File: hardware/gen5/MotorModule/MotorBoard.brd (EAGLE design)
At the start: 61 x 50.1 mm, 42 parts, among them J1 M20X2SHROUDED

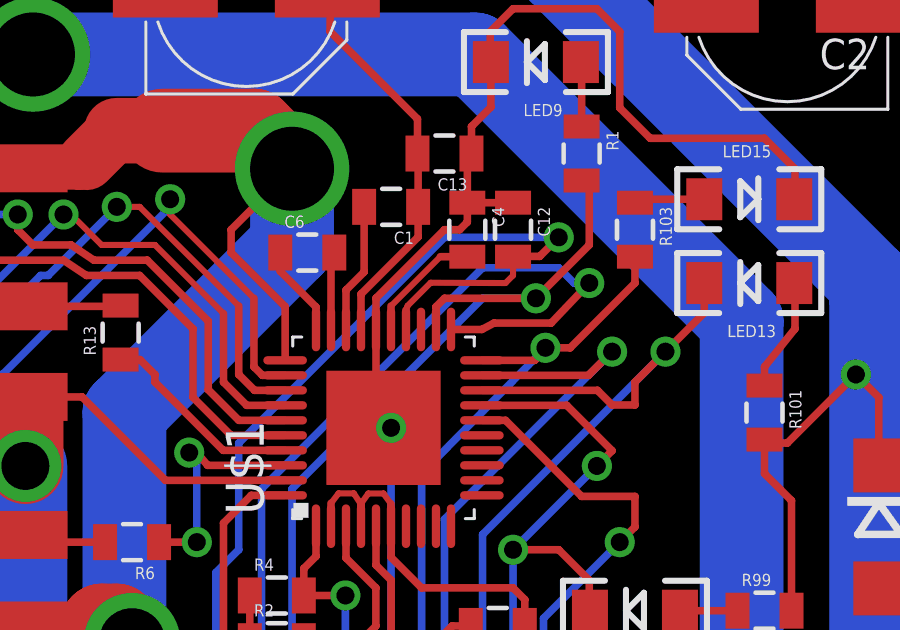
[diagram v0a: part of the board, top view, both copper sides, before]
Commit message: small tweak to motorboard
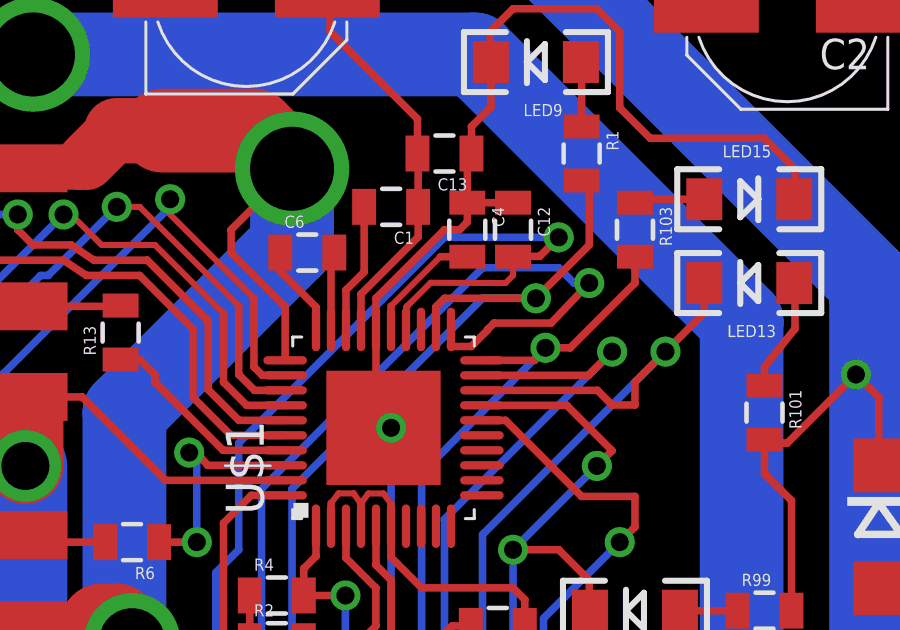
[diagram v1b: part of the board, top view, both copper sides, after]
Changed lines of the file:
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@@
 <wire x1="16.51" y1="36.83" x2="16.51" y2="42.672" width="3.81" layer="1"/>
 <via x="16.51" y="42.672" extent="1-16" drill="2.8"/>
-<wire x1="41.16" y1="33.759" x2="41.16" y2="34.937" width="0.254" layer="1"/>
 <wire x1="41.16" y1="34.937" x2="43.064" y2="36.841" width="0.254" layer="1"/>
 <wire x1="43.064" y1="36.841" x2="43.064" y2="37.846" width="0.254" layer="1"/>
@@
 <wire x1="54.61" y1="29.972" x2="55.372" y2="29.972" width="0.254" layer="1"/>
 <wire x1="55.372" y1="29.972" x2="57.658" y2="32.258" width="0.254" layer="1"/>
+<wire x1="41.16" y1="33.759" x2="41.16" y2="34.937" width="0.254" layer="1"/>
 </signal>
 <signal name="M1O1">
@@
 <wire x1="48.768" y1="35.306" x2="47.498" y2="33.9725" width="0.254" layer="1"/>
 <wire x1="47.498" y1="33.9725" x2="45.593" y2="33.9725" width="0.254" layer="1"/>
-<wire x1="45.593" y1="33.9725" x2="45.189" y2="33.759" width="0.254" layer="1"/>
-<wire x1="45.189" y1="33.759" x2="44.16" y2="33.759" width="0.254" layer="1"/>
 <wire x1="33.274" y1="9.144" x2="26.416" y2="9.144" width="0.254" layer="16"/>
 <wire x1="26.416" y1="9.144" x2="24.13" y2="6.35" width="0.254" layer="16"/>
@@
 <wire x1="36.83" y1="20.066" x2="37.846" y2="21.082" width="0.254" layer="16"/>
 <wire x1="37.846" y1="21.082" x2="37.846" y2="28.448" width="0.254" layer="16"/>
+<wire x1="45.3795" y1="33.759" x2="45.593" y2="33.9725" width="0.254" layer="1"/>
+<wire x1="45.3795" y1="33.759" x2="45.3795" y2="33.740228125" width="0.254" layer="1"/>
+<wire x1="45.3795" y1="33.740228125" x2="44.83100625" y2="33.191734375" width="0.254" layer="1"/>
+<wire x1="44.83100625" y1="33.191734375" x2="44.1569125" y2="33.191734375" width="0.254" layer="1"/>
+<wire x1="44.1569125" y1="33.191734375" x2="44.141415625" y2="33.20723125" width="0.254" layer="1"/>
+<wire x1="44.141415625" y1="33.20723125" x2="44.141415625" y2="33.740415625" width="0" layer="19" extent="1-16"/>
+<wire x1="44.141415625" y1="33.740415625" x2="44.16" y2="33.759" width="0" layer="19" extent="1-16"/>
 </signal>
 <signal name="N$22">
@@
 <wire x1="39.878" y1="18.796" x2="39.116" y2="19.558" width="0.254" layer="1"/>
 <wire x1="39.116" y1="19.558" x2="37.846" y2="19.558" width="0.254" layer="1"/>
-<wire x1="42.66" y1="33.759" x2="42.66" y2="34.405" width="0.254" layer="1"/>
 <wire x1="43.480784375" y1="35.316290625" x2="45.974" y2="35.306" width="0.2032" layer="1"/>
 <wire x1="45.974" y1="35.306" x2="46.228" y2="35.56" width="0.2032" layer="1"/>
@@
 <wire x1="42.66" y1="34.405" x2="42.66030625" y2="34.40530625" width="0.2032" layer="1"/>
 <wire x1="42.66030625" y1="34.40530625" x2="42.7151875" y2="34.55069375" width="0.2032" layer="1"/>
-<wire x1="42.7151875" y1="34.55069375" x2="43.480784375" y2="35.316290625" width="0.2032" layer="1"/>
+<wire x1="42.7151875" y1="34.55069375" x2="42.7964375" y2="34.63194375" width="0.2032" layer="1"/>
 <contactref element="R9" pad="2"/>
+<wire x1="42.7964375" y1="34.63194375" x2="43.480784375" y2="35.316290625" width="0.2032" layer="1"/>
 <wire x1="39.878" y1="14.478" x2="40.654153125" y2="14.478" width="0.2032" layer="1"/>
 <wire x1="40.654153125" y1="14.478" x2="41.562625" y2="13.569528125" width="0.2032" layer="1"/>
 <wire x1="41.562625" y1="13.569528125" x2="42.45130625" y2="13.569528125" width="0.2032" layer="1"/>
 <wire x1="42.45130625" y1="13.569528125" x2="42.49169375" y2="13.529140625" width="0.2032" layer="1"/>
+<wire x1="42.66" y1="33.759" x2="42.66" y2="34.49550625" width="0.2032" layer="1"/>
+<wire x1="42.66" y1="34.49550625" x2="42.7151875" y2="34.55069375" width="0.2032" layer="1"/>
 </signal>
 <signal name="LOCKN">
